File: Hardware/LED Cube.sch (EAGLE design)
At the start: 210 parts, among them IC1 MEGA8-AI, IC10 FT232RL, IC11 FM24V10, IC12 MSGEQ7, IC14 MEGA32-A, IC2 74HC573D, IC3 74HC573D, IC4 74HC573D, IC5 74HC573D, IC6 74HC573D, IC7 74HC573D, IC8 74HC573D, IC9 74HC573D, X2 USB-B-MINI-SMD

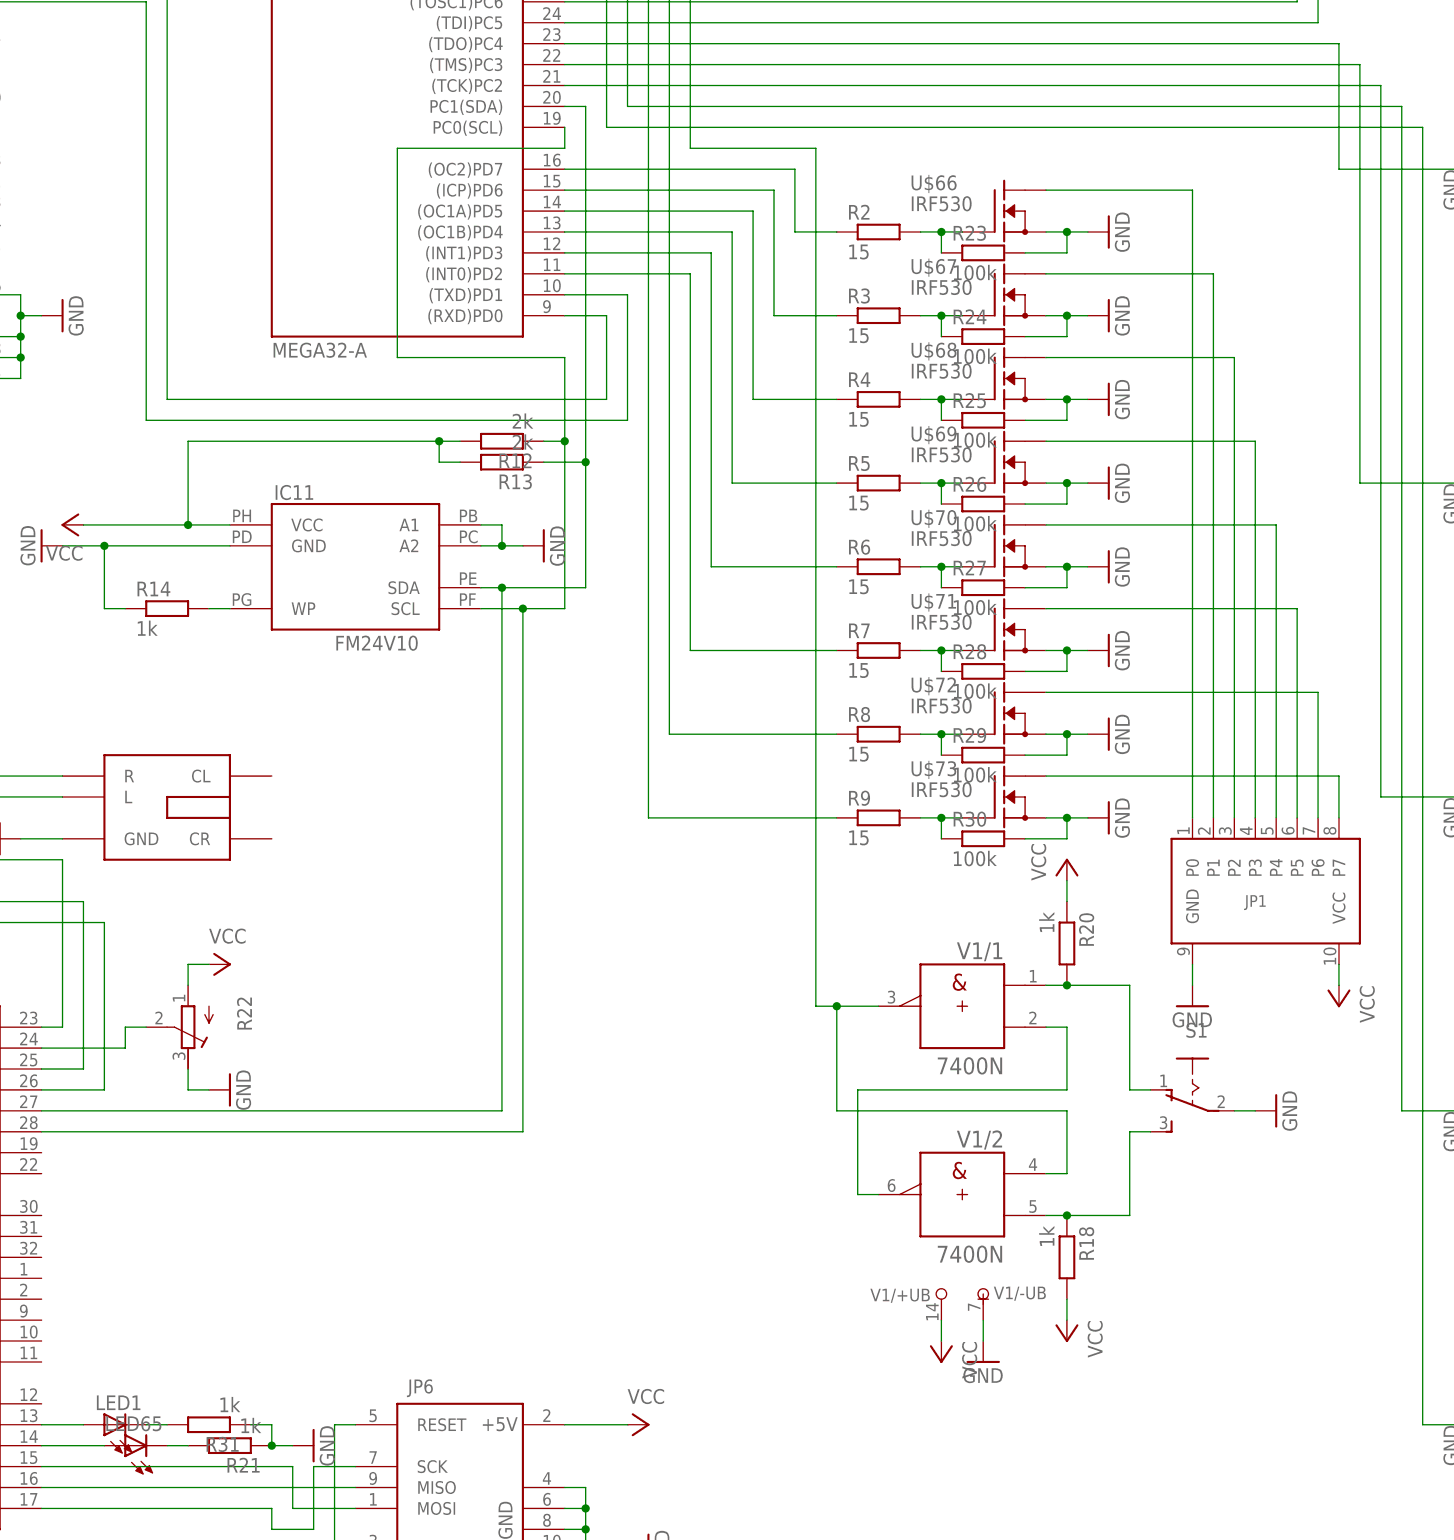
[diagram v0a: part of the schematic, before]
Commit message: Worked at Layout
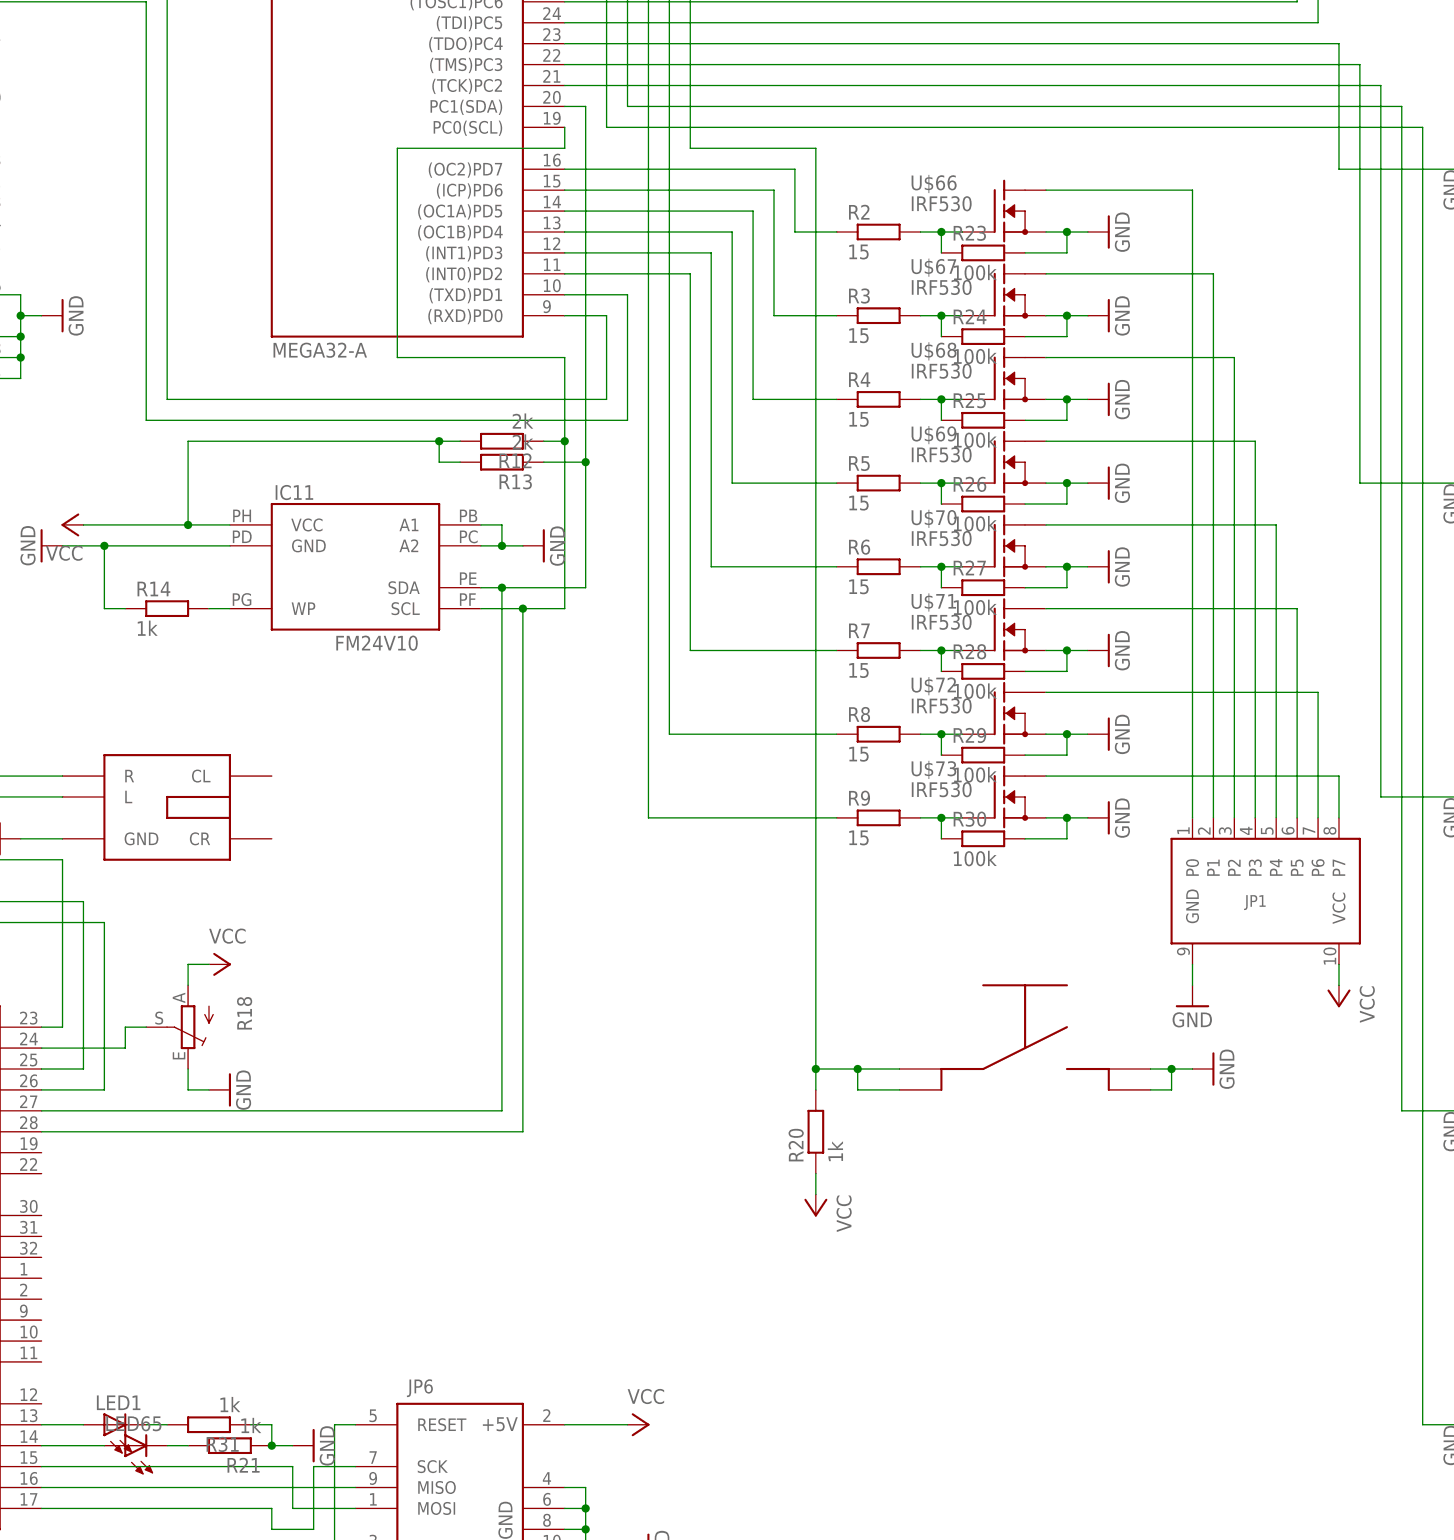
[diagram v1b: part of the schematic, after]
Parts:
- removed R22: (no value), resistor:R-TRIMM3296W
- removed S1: (no value), switch:255SB
- removed V1: 7400N, 74ttl-din:7400N
- added U$74: TASTER, 0-xythobuz:TASTER
- R18: value 1k -> (none); device resistor:R-EU_R0603 -> pot:TRIM_EU-PT10S
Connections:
- removed net N$72: V1/1.B, V1/2.Y
- removed net N$73: R18.1, S1.S, V1/2.B
- removed net N$74: R20.2, S1.O, V1/1.A
- net GND: now also R18.E, U$74.B, U$74.B2; no longer R22.A, S1.P, V1/-UB.-UB
- net N$69: now also R20.2, U$74.A, U$74.A2; no longer V1/1.Y, V1/2.A
- net N$77: now also R18.S; no longer R22.S
- net VCC: now also R18.A; no longer R18.2, R22.E, V1/+UB.+UB
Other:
- moved on the sheet: R20
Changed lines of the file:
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@@
 <part name="R17" library="resistor" deviceset="R-EU_" device="R0603" value="200k"/>
 <part name="GND29" library="supply1" deviceset="GND" device=""/>
-<part name="V1" library="74ttl-din" deviceset="74*00" device="N"/>
-<part name="R18" library="resistor" deviceset="R-EU_" device="R0603" value="1k"/>
 <part name="R20" library="resistor" deviceset="R-EU_" device="R0603" value="1k"/>
-<part name="S1" library="switch" deviceset="255SB" device=""/>
-<part name="P+10" library="supply1" deviceset="VCC" device=""/>
 <part name="P+11" library="supply1" deviceset="VCC" device=""/>
 <part name="GND31" library="supply1" deviceset="GND" device=""/>
@@
 <part name="R21" library="resistor" deviceset="R-EU_" device="R0603" value="1k"/>
 <part name="GND36" library="supply1" deviceset="GND" device=""/>
-<part name="R22" library="resistor" deviceset="R-TRIMM" device="3296W"/>
 <part name="GND37" library="supply1" deviceset="GND" device=""/>
 <part name="P+14" library="supply1" deviceset="VCC" device=""/>
@@
 <part name="GND39" library="supply1" deviceset="GND" device=""/>
 <part name="P+79" library="supply1" deviceset="VCC" device=""/>
-<part name="GND40" library="supply1" deviceset="GND" device=""/>
-<part name="P+80" library="supply1" deviceset="VCC" device=""/>
 <part name="U$66" library="0-xythobuz" deviceset="IRF530" device=""/>
 <part name="U$67" library="0-xythobuz" deviceset="IRF530" device=""/>
@@
 <part name="U$72" library="0-xythobuz" deviceset="IRF530" device=""/>
 <part name="U$73" library="0-xythobuz" deviceset="IRF530" device=""/>
+<part name="U$74" library="0-xythobuz" deviceset="TASTER" device=""/>
+<part name="R18" library="pot" deviceset="TRIM_EU-" device="PT10S"/>
 </parts>
 <sheets>
@@
 <instance part="R17" gate="G$1" x="-38.1" y="-50.8" rot="R180"/>
 <instance part="GND29" gate="1" x="-30.48" y="-53.34" rot="R270"/>
-<instance part="V1" gate="/1" x="86.36" y="-73.66" rot="MR0"/>
-<instance part="V1" gate="/2" x="86.36" y="-96.52" rot="MR0"/>
-<instance part="R18" gate="G$1" x="99.06" y="-104.14" rot="R270"/>
-<instance part="R20" gate="G$1" x="99.06" y="-66.04" rot="R270"/>
-<instance part="S1" gate="1" x="114.3" y="-83.82" rot="MR270"/>
-<instance part="P+10" gate="VCC" x="99.06" y="-114.3" rot="R180"/>
-<instance part="P+11" gate="VCC" x="99.06" y="-55.88"/>
-<instance part="GND31" gate="1" x="124.46" y="-86.36" rot="R90"/>
+<instance part="R20" gate="G$1" x="68.58" y="-88.9" rot="R90"/>
+<instance part="P+11" gate="VCC" x="68.58" y="-99.06" rot="R180"/>
+<instance part="GND31" gate="1" x="116.84" y="-81.28" rot="R90"/>
 <instance part="R19" gate="G$1" x="-83.82" y="-76.2" rot="R180"/>
 <instance part="Q10" gate="G$1" x="-78.74" y="-96.52" rot="R90"/>
@@
 <instance part="R21" gate="G$1" x="-2.54" y="-127" rot="R180"/>
 <instance part="GND36" gate="1" x="7.62" y="-127" rot="R90"/>
-<instance part="R22" gate="G$1" x="-7.62" y="-76.2" rot="R180"/>
 <instance part="GND37" gate="1" x="-2.54" y="-83.82" rot="R90"/>
 <instance part="P+14" gate="VCC" x="-2.54" y="-68.58" rot="R270"/>
@@
 <instance part="GND39" gate="1" x="114.3" y="-73.66"/>
 <instance part="P+79" gate="VCC" x="132.08" y="-73.66" rot="R180"/>
-<instance part="V1" gate="/+UB" x="83.82" y="-109.22" rot="R180"/>
-<instance part="V1" gate="/-UB" x="88.9" y="-109.22"/>
-<instance part="GND40" gate="1" x="88.9" y="-116.84"/>
-<instance part="P+80" gate="VCC" x="83.82" y="-116.84" rot="R180"/>
 <instance part="U$66" gate="G$1" x="91.44" y="22.86"/>
 <instance part="U$67" gate="G$1" x="91.44" y="12.7"/>
@@
 <instance part="U$72" gate="G$1" x="91.44" y="-38.1"/>
 <instance part="U$73" gate="G$1" x="91.44" y="-48.26"/>
+<instance part="U$74" gate="G$1" x="93.98" y="-81.28"/>
+<instance part="R18" gate="1" x="-7.62" y="-76.2" rot="R180"/>
 </instances>
 <busses>
@@
 </segment>
 <segment>
-<wire x1="121.92" y1="-86.36" x2="119.38" y2="-86.36" width="0.1524" layer="91"/>
-<pinref part="GND31" gate="1" pin="GND"/>
-<pinref part="S1" gate="1" pin="P"/>
-</segment>
-<segment>
 <wire x1="-91.44" y1="-93.98" x2="-93.98" y2="-93.98" width="0.1524" layer="91"/>
 <wire x1="-93.98" y1="-93.98" x2="-93.98" y2="-96.52" width="0.1524" layer="91"/>
@@
 <wire x1="-7.62" y1="-83.82" x2="-7.62" y2="-81.28" width="0.1524" layer="91"/>
 <pinref part="GND37" gate="1" pin="GND"/>
-<pinref part="R22" gate="G$1" pin="A"/>
+<pinref part="R18" gate="1" pin="E"/>
 </segment>
 <segment>
@@
 </segment>
 <segment>
-<pinref part="GND40" gate="1" pin="GND"/>
-<pinref part="V1" gate="/-UB" pin="-UB"/>
-<wire x1="88.9" y1="-114.3" x2="88.9" y2="-111.76" width="0.1524" layer="91"/>
+<pinref part="U$74" gate="G$1" pin="B"/>
+<pinref part="GND31" gate="1" pin="GND"/>
+<wire x1="109.22" y1="-81.28" x2="111.76" y2="-81.28" width="0.1524" layer="91"/>
+<pinref part="U$74" gate="G$1" pin="B2"/>
+<wire x1="111.76" y1="-81.28" x2="114.3" y2="-81.28" width="0.1524" layer="91"/>
+<wire x1="109.22" y1="-83.82" x2="111.76" y2="-83.82" width="0.1524" layer="91"/>
+<wire x1="111.76" y1="-83.82" x2="111.76" y2="-81.28" width="0.1524" layer="91"/>
+<junction x="111.76" y="-81.28"/>
 </segment>
 </net>
@@
 </segment>
 <segment>
-<wire x1="99.06" y1="-111.76" x2="99.06" y2="-109.22" width="0.1524" layer="91"/>
-<pinref part="P+10" gate="VCC" pin="VCC"/>
-<pinref part="R18" gate="G$1" pin="2"/>
-</segment>
-<segment>
-<wire x1="99.06" y1="-60.96" x2="99.06" y2="-58.42" width="0.1524" layer="91"/>
+<wire x1="68.58" y1="-93.98" x2="68.58" y2="-96.52" width="0.1524" layer="91"/>
 <pinref part="R20" gate="G$1" pin="1"/>
 <pinref part="P+11" gate="VCC" pin="VCC"/>
@@
 <wire x1="-7.62" y1="-68.58" x2="-7.62" y2="-71.12" width="0.1524" layer="91"/>
 <pinref part="P+14" gate="VCC" pin="VCC"/>
-<pinref part="R22" gate="G$1" pin="E"/>
+<pinref part="R18" gate="1" pin="A"/>
 </segment>
 <segment>
@@
 <pinref part="JP1" gate="G$1" pin="VCC"/>
 <wire x1="132.08" y1="-71.12" x2="132.08" y2="-68.58" width="0.1524" layer="91"/>
-</segment>
-<segment>
-<pinref part="P+80" gate="VCC" pin="VCC"/>
-<pinref part="V1" gate="/+UB" pin="+UB"/>
-<wire x1="83.82" y1="-114.3" x2="83.82" y2="-111.76" width="0.1524" layer="91"/>
 </segment>
 </net>
@@
 <wire x1="53.34" y1="55.88" x2="38.1" y2="55.88" width="0.1524" layer="91"/>
 <wire x1="68.58" y1="30.48" x2="53.34" y2="30.48" width="0.1524" layer="91"/>
-<wire x1="76.2" y1="-73.66" x2="71.12" y2="-73.66" width="0.1524" layer="91"/>
-<wire x1="71.12" y1="-73.66" x2="68.58" y2="-73.66" width="0.1524" layer="91"/>
-<wire x1="68.58" y1="30.48" x2="68.58" y2="-73.66" width="0.1524" layer="91"/>
-<wire x1="96.52" y1="-93.98" x2="99.06" y2="-93.98" width="0.1524" layer="91"/>
-<wire x1="99.06" y1="-93.98" x2="99.06" y2="-86.36" width="0.1524" layer="91"/>
-<wire x1="99.06" y1="-86.36" x2="71.12" y2="-86.36" width="0.1524" layer="91"/>
-<wire x1="71.12" y1="-86.36" x2="71.12" y2="-73.66" width="0.1524" layer="91"/>
-<junction x="71.12" y="-73.66"/>
-<pinref part="V1" gate="/1" pin="Y"/>
-<pinref part="V1" gate="/2" pin="A"/>
+<wire x1="78.74" y1="-81.28" x2="73.66" y2="-81.28" width="0.1524" layer="91"/>
+<wire x1="73.66" y1="-81.28" x2="68.58" y2="-81.28" width="0.1524" layer="91"/>
+<wire x1="68.58" y1="30.48" x2="68.58" y2="-81.28" width="0.1524" layer="91"/>
 <pinref part="IC14" gate="G$1" pin="(T0/XCK)PB0"/>
-</segment>
-</net>
-<net name="N$72" class="0">
-<segment>
-<wire x1="76.2" y1="-96.52" x2="73.66" y2="-96.52" width="0.1524" layer="91"/>
-<wire x1="73.66" y1="-96.52" x2="73.66" y2="-83.82" width="0.1524" layer="91"/>
-<wire x1="73.66" y1="-83.82" x2="99.06" y2="-83.82" width="0.1524" layer="91"/>
-<wire x1="99.06" y1="-83.82" x2="99.06" y2="-76.2" width="0.1524" layer="91"/>
-<wire x1="99.06" y1="-76.2" x2="96.52" y2="-76.2" width="0.1524" layer="91"/>
-<pinref part="V1" gate="/2" pin="Y"/>
-<pinref part="V1" gate="/1" pin="B"/>
-</segment>
-</net>
-<net name="N$73" class="0">
-<segment>
-<wire x1="96.52" y1="-99.06" x2="99.06" y2="-99.06" width="0.1524" layer="91"/>
-<wire x1="99.06" y1="-99.06" x2="106.68" y2="-99.06" width="0.1524" layer="91"/>
-<wire x1="106.68" y1="-99.06" x2="106.68" y2="-88.9" width="0.1524" layer="91"/>
-<wire x1="106.68" y1="-88.9" x2="109.22" y2="-88.9" width="0.1524" layer="91"/>
-<junction x="99.06" y="-99.06"/>
-<pinref part="V1" gate="/2" pin="B"/>
-<pinref part="R18" gate="G$1" pin="1"/>
-<pinref part="S1" gate="1" pin="S"/>
-</segment>
-</net>
-<net name="N$74" class="0">
-<segment>
-<wire x1="109.22" y1="-83.82" x2="106.68" y2="-83.82" width="0.1524" layer="91"/>
-<wire x1="106.68" y1="-83.82" x2="106.68" y2="-71.12" width="0.1524" layer="91"/>
-<wire x1="106.68" y1="-71.12" x2="99.06" y2="-71.12" width="0.1524" layer="91"/>
-<wire x1="96.52" y1="-71.12" x2="99.06" y2="-71.12" width="0.1524" layer="91"/>
-<junction x="99.06" y="-71.12"/>
-<pinref part="S1" gate="1" pin="O"/>
 <pinref part="R20" gate="G$1" pin="2"/>
-<pinref part="V1" gate="/1" pin="A"/>
+<wire x1="68.58" y1="-83.82" x2="68.58" y2="-81.28" width="0.1524" layer="91"/>
+<junction x="68.58" y="-81.28"/>
+<pinref part="U$74" gate="G$1" pin="A"/>
+<pinref part="U$74" gate="G$1" pin="A2"/>
+<wire x1="78.74" y1="-83.82" x2="73.66" y2="-83.82" width="0.1524" layer="91"/>
+<wire x1="73.66" y1="-83.82" x2="73.66" y2="-81.28" width="0.1524" layer="91"/>
+<junction x="73.66" y="-81.28"/>
 </segment>
 </net>
@@
 <wire x1="-15.24" y1="-78.74" x2="-15.24" y2="-76.2" width="0.1524" layer="91"/>
 <wire x1="-15.24" y1="-76.2" x2="-12.7" y2="-76.2" width="0.1524" layer="91"/>
-<pinref part="R22" gate="G$1" pin="S"/>
 <pinref part="IC1" gate="G$1" pin="PC1(ADC1)"/>
-</segment>
-</net>
+<pinref part="R18" gate="1" pin="S"/>
+</segment>
+</net>
